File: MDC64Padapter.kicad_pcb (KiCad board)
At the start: 2 copper layers, 33 parts, among them J1 DB9_F_TO_C64, J2 DB9_M_TO_PAD, Q1 BC847, Q2 BC847, SW1 MODE, U1 74ACT08, U2 74ACT373, U3 74ACT157, U4 74ACT373, U6 NE555D

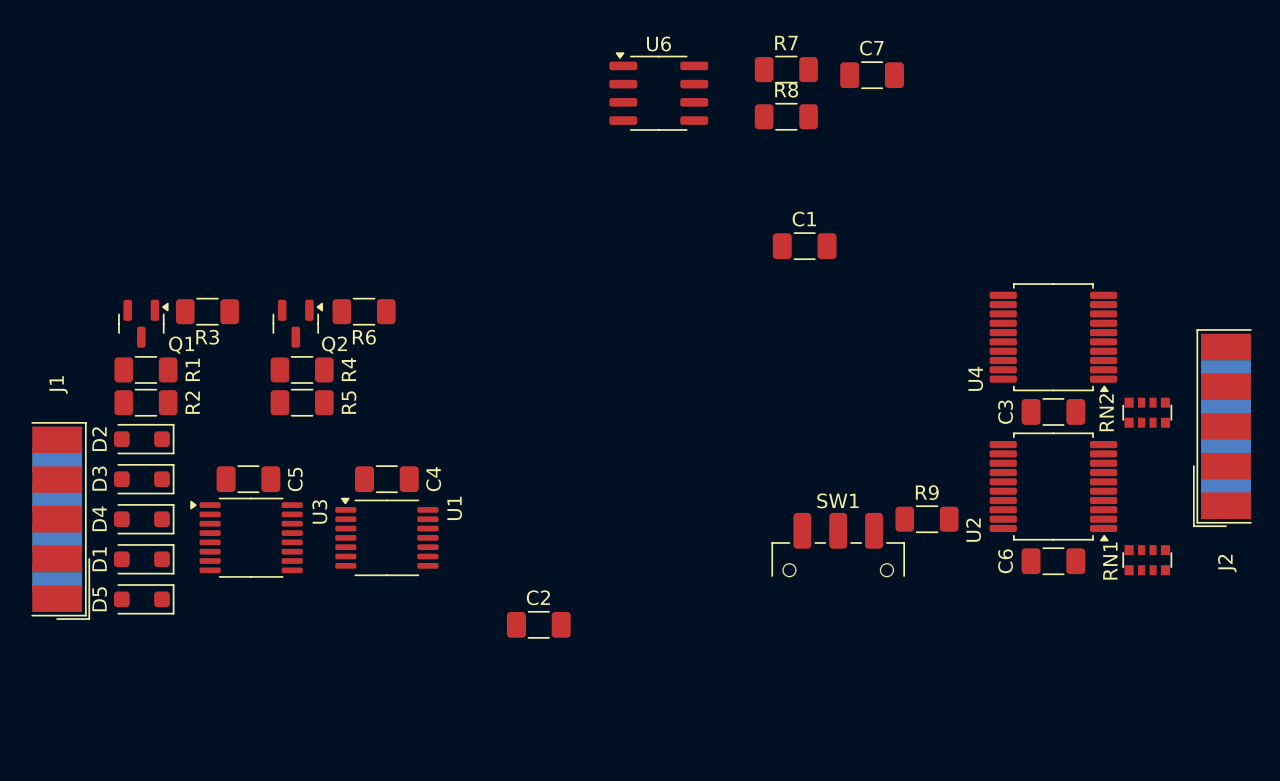
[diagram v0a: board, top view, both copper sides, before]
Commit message: Reorganize pcb a bit
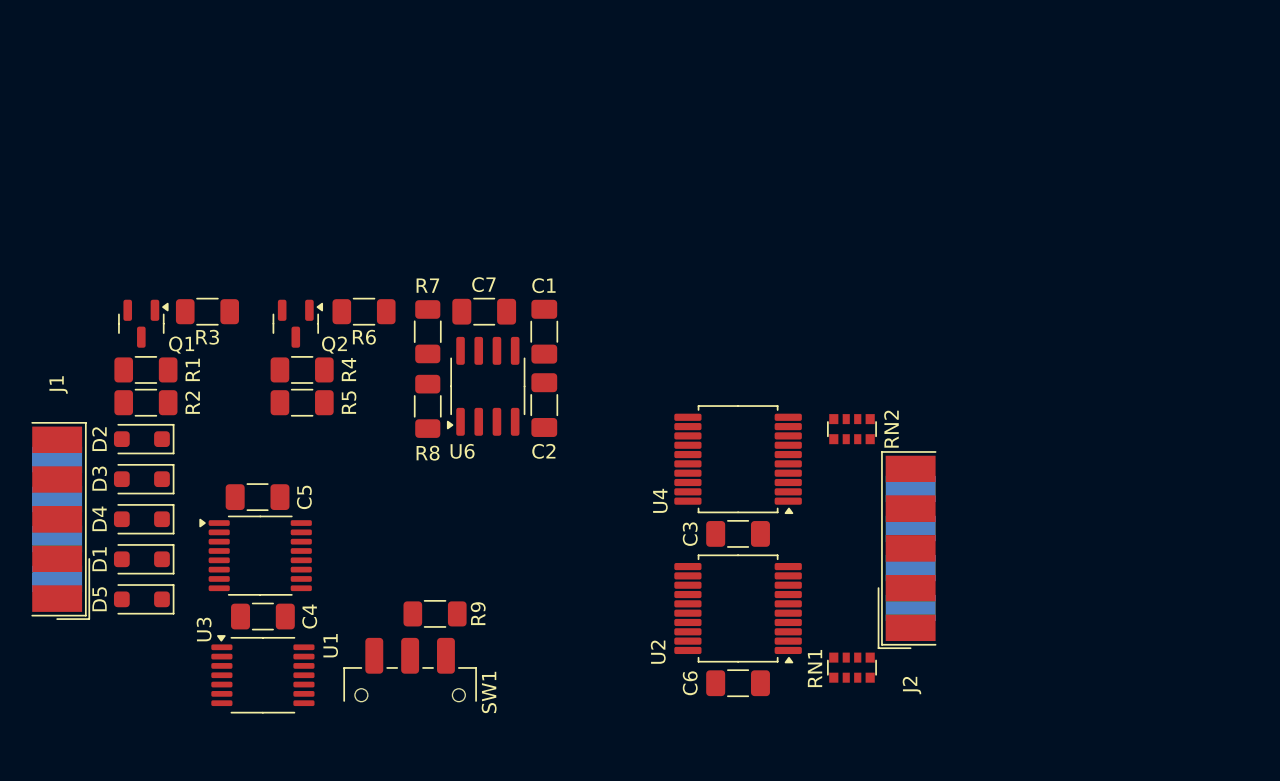
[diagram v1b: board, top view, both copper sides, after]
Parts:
- moved R9 34.9 mm to (83.2, 122.9)
- moved R8 32.2 mm to (82.7, 108.5), turned to -90 degrees
- moved C7 31.7 mm to (86.6, 101.9)
- moved SW1 31.1 mm to (81.4, 128.6)
- moved R7 31.0 mm to (82.7, 103.3), turned to -90 degrees
- moved U6 23.7 mm to (86.9, 107.1), turned to 90 degrees
- moved J2 23.6 mm to (116.4, 118.4)
- moved C3 23.6 mm to (104.3, 117.4)
- moved C6 23.6 mm to (104.3, 127.8)
- moved U2 23.6 mm to (104.3, 122.6)
- moved U4 23.6 mm to (104.3, 112.1)
- moved RN1 21.9 mm to (112.3, 126.7)
- moved RN2 20.6 mm to (112.3, 110.0), turned to -90 degrees
- moved C1 19.1 mm to (90.8, 103.3), turned to -90 degrees
- moved C2 15.3 mm to (90.8, 108.4), turned to 90 degrees
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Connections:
- RN1 pad 1: GND -> unconnected-(RN1-R1.1-Pad1)
- RN1 pad 2: GND -> VCC
- RN1 pad 3: GND -> VCC
- RN1 pad 4: GND -> VCC
- RN1 pad 5: /MD_RIGHT_M -> /C64_UP
- RN1 pad 6: /MD_LEFT_M -> /MD_B/~{A}
- RN1 pad 7: /MD_B/~{A} -> /C64_DOWN
- RN1 pad 8: /MD_C/~{ST} -> /MD_LEFT_M
- RN2 pad 1: GND -> VCC
- RN2 pad 2: GND -> VCC
- RN2 pad 3: GND -> VCC
- RN2 pad 4: GND -> VCC
- RN2 pad 7: /MD_B/~{A} -> /MD_RIGHT_M

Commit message: First PCB design
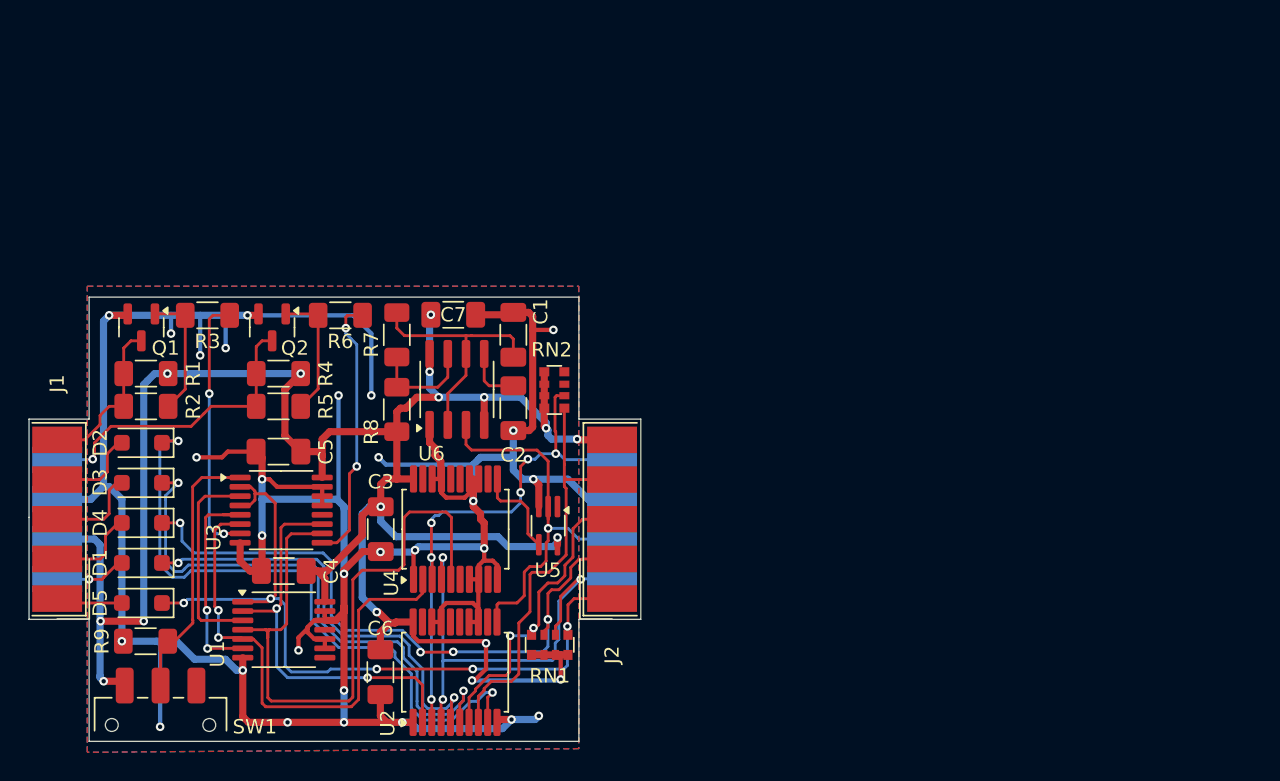
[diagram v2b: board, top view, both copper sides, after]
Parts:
- added U5: 74AHC1G04, Package_TO_SOT_SMD:SOT-353_SC-70-5_Handsoldering, F.Cu at (91.1, 116.8)
- moved C6 25.0 mm to (79.4, 127.0), turned to -90 degrees
- moved C3 24.9 mm to (79.4, 117.0), turned to -90 degrees
- moved RN1 21.1 mm to (91.2, 125.1)
- moved RN2 20.9 mm to (91.5, 107.3), turned to 0 degrees
- moved J2 20.9 mm to (95.5, 116.3)
- moved U4 20.3 mm to (84.6, 117.0), turned to 90 degrees
- moved R9 20.3 mm to (63.0, 124.8), turned to 180 degrees
- moved U2 20.2 mm to (84.6, 127.0), turned to 90 degrees
- moved SW1 17.5 mm to (64.0, 130.7)
- moved C5 3.49 mm to (72.3, 111.6)
- moved U3 3.49 mm to (72.5, 115.7)
- moved C4 3.49 mm to (72.6, 119.9)
- moved U1 3.49 mm to (72.6, 124.0)
- moved C7 2.17 mm to (84.5, 102.1)
- moved R8 2.17 mm to (80.5, 108.7)
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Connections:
- RN1 pad 1: unconnected-(RN1-R1.1-Pad1) -> VCC
- RN2 pad 5: unconnected-(RN2-R4.2-Pad5) -> /MD_RIGHT_M
- RN2 pad 6: unconnected-(RN2-R3.2-Pad6) -> /MD_C/~{ST}
- RN2 pad 7: /MD_RIGHT_M -> unconnected-(RN2-R2.2-Pad7)
- RN2 pad 8: /MD_C/~{ST} -> unconnected-(RN2-R1.2-Pad8)
- U1 pad 6: Net-(U3-I0c) -> Net-(U3-I0b)
- U3 pad 10: /MD_START -> /MD_A
- U3 pad 11: Net-(U3-I0c) -> /MD_C
- U3 pad 5: /MD_C -> Net-(U3-I0b)
- U3 pad 6: /MD_A -> /MD_START
- U3 pad 7: /C64_B -> /C64_C
- U3 pad 9: /C64_C -> /C64_B
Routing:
- net GND: track 0.00 -> 244.0 mm, vias 0 -> 29
- net VCC: track 0.00 -> 159.1 mm, vias 0 -> 17
- net /C64_UP: track 0.00 -> 54.8 mm, vias 0 -> 5
- net /MD_A: track 0.00 -> 47.3 mm
- net /C64_RIGHT: track 0.00 -> 45.5 mm, vias 0 -> 2
- net /C64_DOWN: track 0.00 -> 44.9 mm, vias 0 -> 4
- net /C64_LEFT: track 0.00 -> 39.8 mm, vias 0 -> 2
- net /MD_C/~{ST}: track 0.00 -> 36.5 mm, vias 0 -> 6
- net /MD_START: track 0.00 -> 36.0 mm, vias 0 -> 2
- net /MD_B/~{A}: track 0.00 -> 34.2 mm, vias 0 -> 3
- net /C64_FIRE: track 0.00 -> 30.9 mm, vias 0 -> 2
- net /MD_RIGHT_M: track 0.00 -> 29.4 mm
- net /MD_C: track 0.00 -> 28.5 mm, vias 0 -> 2
- net /CLK: track 0.00 -> 27.1 mm, vias 0 -> 1
- net /MD_LEFT_M: track 0.00 -> 21.8 mm, vias 0 -> 2
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- added copper zone on B.Cu, net GND
- added copper zone on F.Cu, net GND
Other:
- board outline added: 42.7 x 31 mm
